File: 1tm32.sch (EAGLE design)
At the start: 38 parts, among them IC1 STM32L412RBT6P, IC2 BGM240PA32VNN3, J1 FTSH-107-01-L-DV-K-A, J2 10118192-0001LF, SW1 LL3301FF065QJ, U2 LD39050PU33R, Y1 8MHz, Y2 32.7KHz

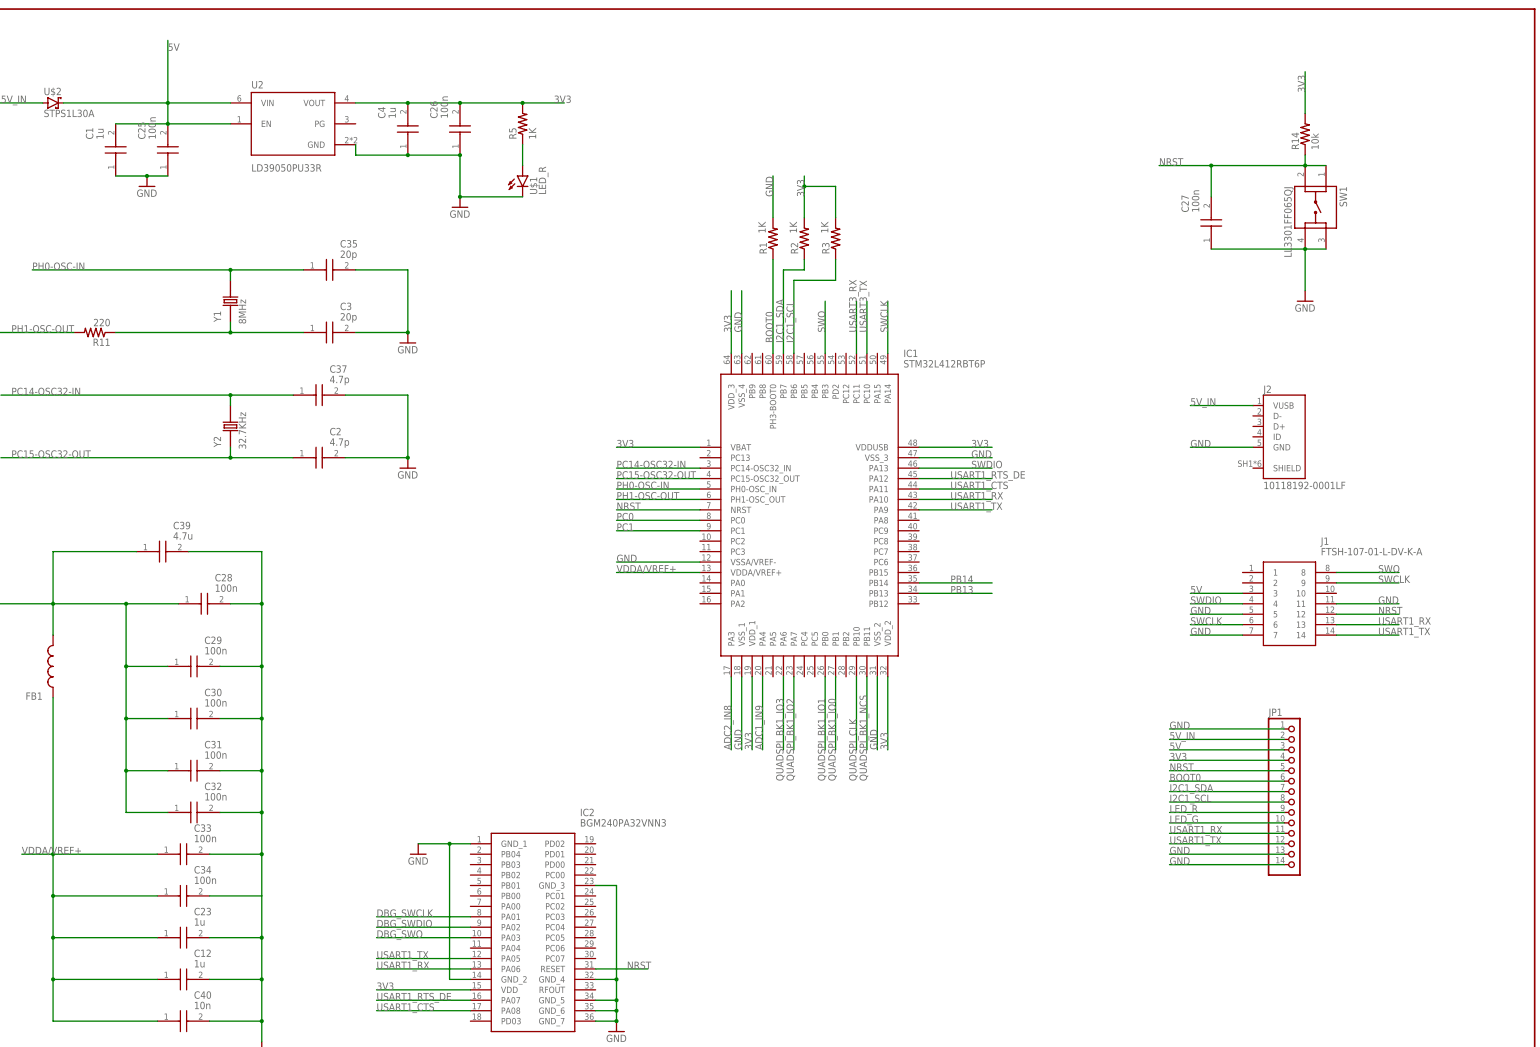
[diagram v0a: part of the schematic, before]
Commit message: layout completed
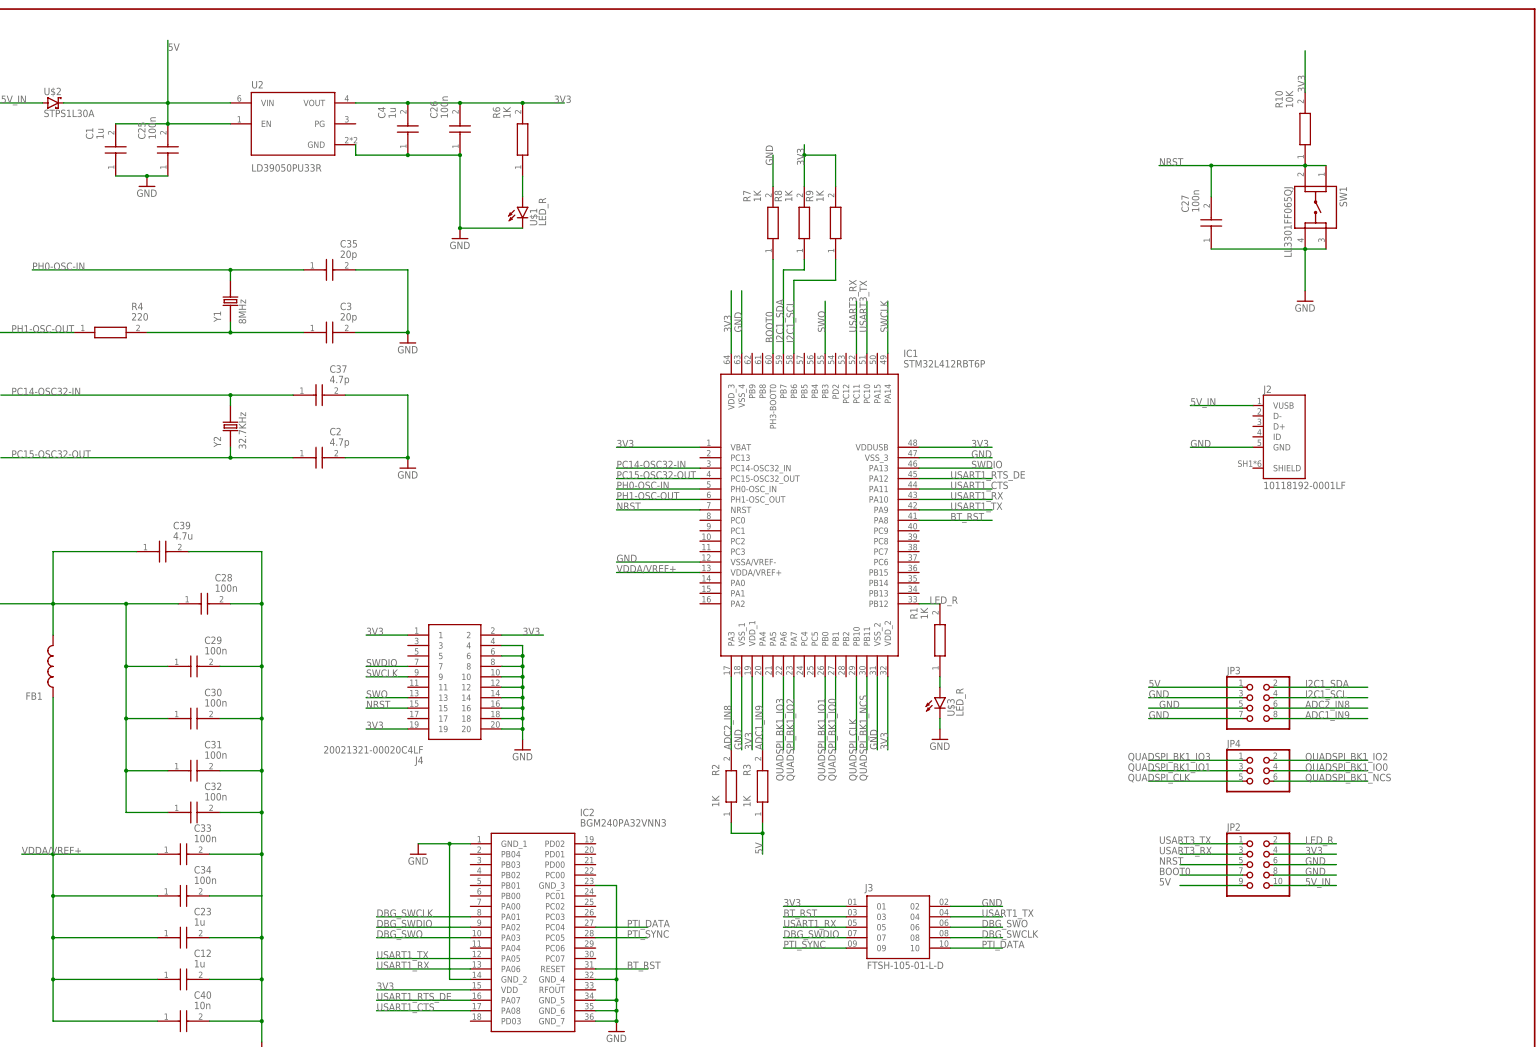
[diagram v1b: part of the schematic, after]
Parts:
- removed J1: FTSH-107-01-L-DV-K-A, ce-capstone:FTSH-107-01-L-DV-K-A
- removed JP1: (no value), pinhead:PINHD-1X14
- removed R11: 220, ce-capstone:RT0402FRE07220RL
- removed R14: 10k, ce-capstone:RC0402FR-0710KL
- removed R5: 1K, ce-capstone:RC0402FR-071KL
- added J3: FTSH-105-01-L-D, FTSH-105-01-L-D(bt_connect):FTSH-105-01-L-D
- added J4: 20021321-00020C4LF, 20021321-00020C4LF(20head):20021321-00020C4LF
- added JP2: (no value), pinhead:PINHD-2X5
- added JP3: (no value), pinhead:PINHD-2X4
- added JP4: (no value), pinhead:PINHD-2X3
- added R10: 10K, RC0805JR-0710KL:RC0805JR-0710KL
- added R4: 220, RC0805FR-10220RL:RC0805FR-10220RL
- added R6, R7, R8, R9: 1K, RC0805FR-131KL:RC0805FR-131KL
- added U$3: LED_R, ce-capstone:SML-P12VTT86
- R1, R2, R3: device ce-capstone:RC0402FR-071KL -> RC0805FR-131KL:RC0805FR-131KL
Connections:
- removed net LED_G: JP1.10
- removed net PB13: IC1.PB13
- removed net PB14: IC1.PB14
- removed net PC0: IC1.PC0
- removed net PC1: IC1.PC1
- new net BT_RST: IC1.PA8, IC2.RESET, J3.03
- new net N$2: R1.1, U$3.A
- new net PTI_DATA: IC2.PC04, J3.10
- new net PTI_SYNC: IC2.PC05, J3.09
- net 3V3: now also J3.01, J4.1, J4.19, J4.2, JP2.4, R10.2, R6.2, R8.2, R9.2; no longer JP1.4, R14.2, R2.2, R3.2, R5.2
- net 5V: now also JP2.9, JP3.1, R2.1, R3.1; no longer J1.3, JP1.3
- net 5V_IN: now also JP2.10; no longer JP1.2
- net ADC1_IN9: now also JP3.8, R3.2
- net ADC2_IN8: now also JP3.6, R2.2
- net BOOT0: now also JP2.7, R7.1; no longer JP1.6, R1.1
- net DBG_SWCLK: now also J3.08
- net DBG_SWDIO: now also J3.07
- net DBG_SWO: now also J3.06
- net GND: now also J3.02, J4.10, J4.12, J4.14, J4.16, J4.18, J4.20, J4.4, J4.6, J4.8, JP2.6, JP2.8, JP3.3, JP3.5, JP3.7, R7.2, U$3.C; no longer J1.11, J1.5, J1.7, JP1.1, JP1.13, JP1.14, R1.2
- net I2C1_SCL: now also JP3.4, R9.1; no longer JP1.8, R3.1
- net I2C1_SDA: now also JP3.2, R8.1; no longer JP1.7, R2.1
- net LED_R: now also IC1.PB12, JP2.2, R1.2; no longer JP1.9
- net N$3: now also R4.2; no longer R11.1
- net N$5: now also R6.1; no longer R5.1
- net NRST: now also J4.15, JP2.5, R10.1; no longer IC2.RESET, J1.12, JP1.5, R14.1
- net PH1-OSC-OUT: now also R4.1; no longer R11.2
- net QUADSPI_BK1_IO0: now also JP4.4
- net QUADSPI_BK1_IO1: now also JP4.3
- net QUADSPI_BK1_IO2: now also JP4.2
- net QUADSPI_BK1_IO3: now also JP4.1
- net QUADSPI_BK1_NCS: now also JP4.6
- net QUADSPI_CLK: now also JP4.5
- net SWCLK: now also J4.9; no longer J1.6, J1.9
- net SWDIO: now also J4.7; no longer J1.4
- net SWO: now also J4.13; no longer J1.8
- net USART1_RX: now also J3.05; no longer J1.13, JP1.11
- net USART1_TX: now also J3.04; no longer J1.14, JP1.12
- net USART3_RX: now also JP2.3
- net USART3_TX: now also JP2.1
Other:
- moved on the sheet: U$1
